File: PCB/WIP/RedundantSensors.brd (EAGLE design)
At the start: 111.7 x 100 mm, 176 parts, among them J1 10118192-0001LF, J3 503182-1852, J4 JST-SH-4_SMT_V, U1 TPD4F003DQDR, U10 LIS3MDLTR, U2 BMI088, U3 BMI088, U4 BMI088, U5 STM32H743ZIT6, U6 LIS3MDLTR, U7 LIS3MDLTR, X1 LiDAR, X2 Telemetry, X3 RC, Y2 8MHz

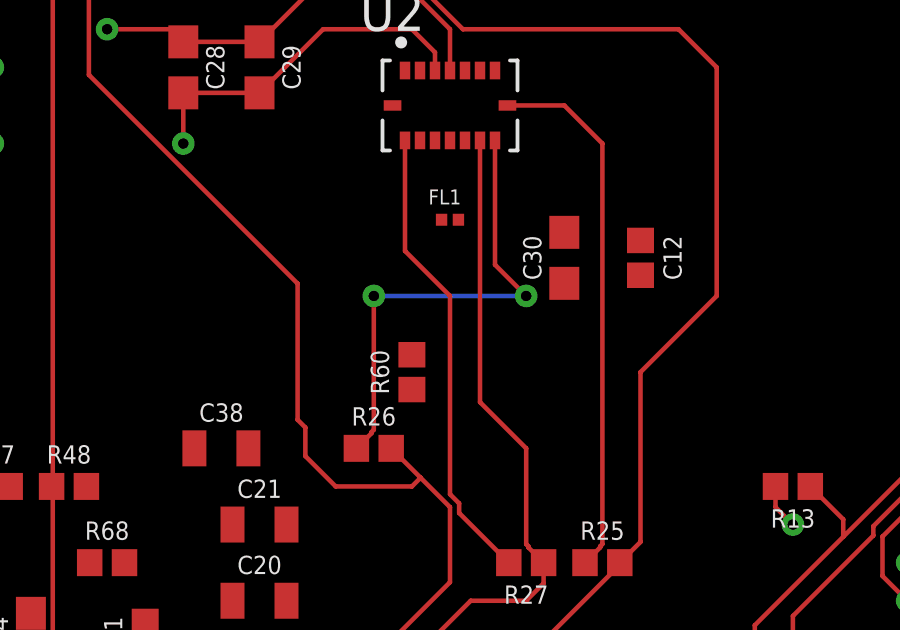
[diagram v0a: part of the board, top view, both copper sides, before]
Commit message: PCB update
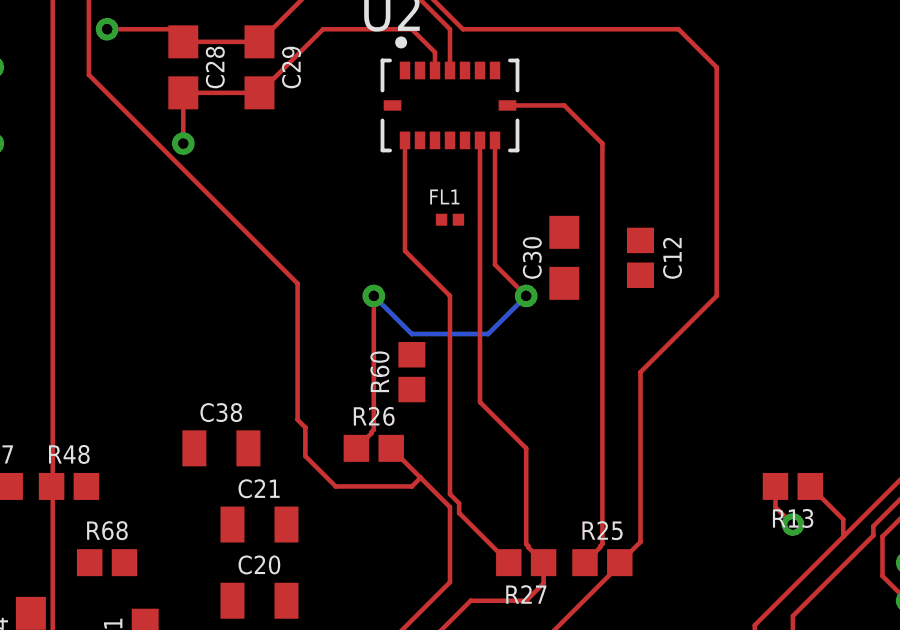
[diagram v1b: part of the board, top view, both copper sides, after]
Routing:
- net N$27: track 16.2 -> 17.2 mm
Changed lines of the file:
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@@
 <wire x1="68.58" y1="74.2782875" x2="68.58" y2="78.74" width="0.1524" layer="1"/>
 <via x="68.58" y="78.74" extent="1-16" drill="0.35"/>
-<wire x1="68.58" y1="78.74" x2="73.66" y2="78.74" width="0.1524" layer="16"/>
+<wire x1="72.39" y1="77.47" x2="69.85" y2="77.47" width="0.1524" layer="16"/>
+<wire x1="68.58" y1="78.74" x2="69.85" y2="77.47" width="0.1524" layer="16"/>
+<wire x1="72.39" y1="77.47" x2="73.66" y2="78.74" width="0.1524" layer="16"/>
 <via x="73.66" y="78.74" extent="1-16" drill="0.35"/>
 <wire x1="73.66" y1="78.74" x2="72.62" y2="79.78" width="0.1524" layer="1"/>
